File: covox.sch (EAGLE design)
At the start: 25 parts, among them CN1 POWERJACK, IC1 74HCT373N, IC2 74HC164N

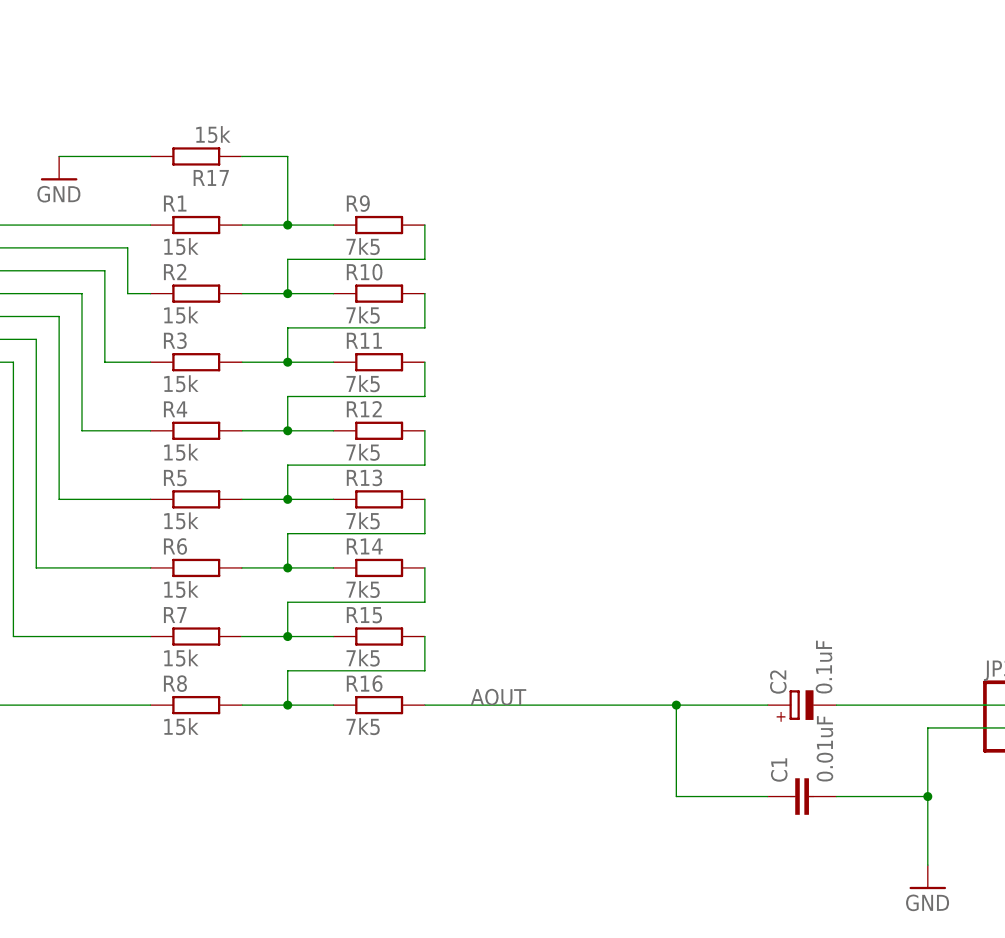
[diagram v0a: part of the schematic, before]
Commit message: Updates...
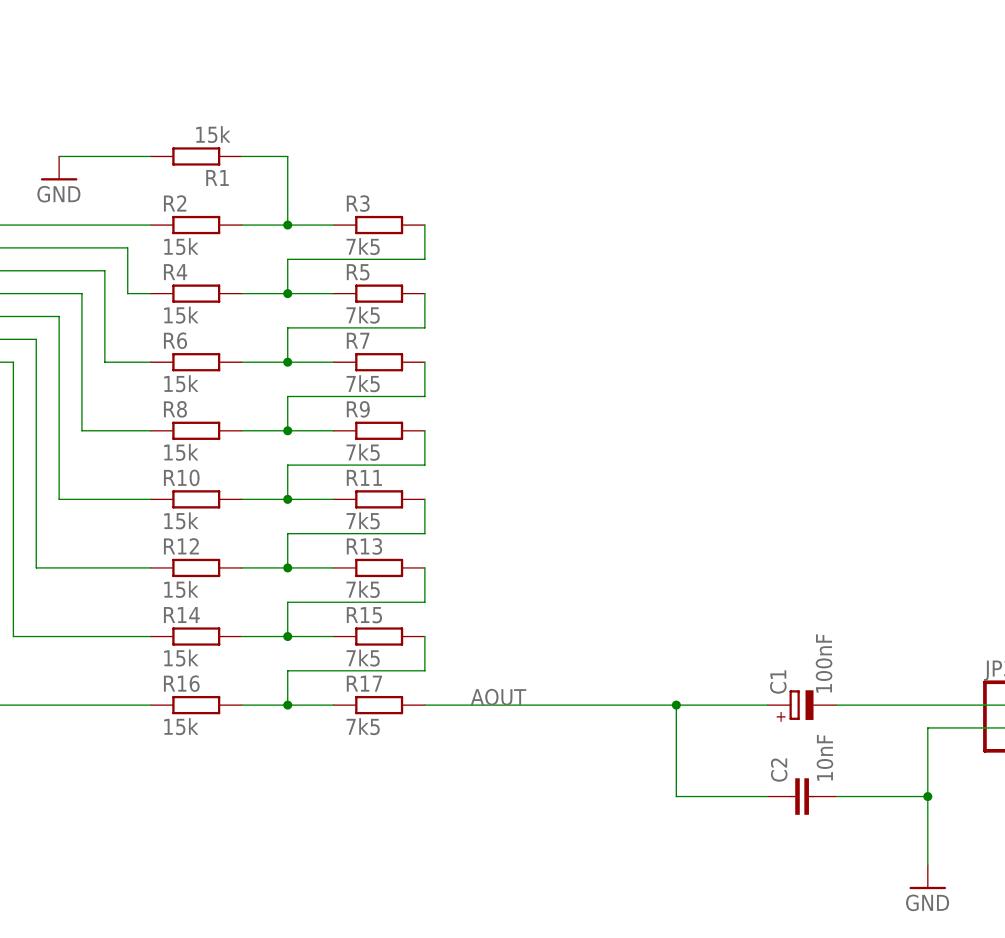
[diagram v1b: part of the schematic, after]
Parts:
- C1: value 0.01uF -> 100nF; device rcl:C-EU025-025X050 -> rcl:CPOL-EUE2-4
- C2: value 0.1uF -> 10nF; device rcl:CPOL-EUE2-4 -> rcl:C-EU025-025X050
- R10, R12, R14, R16: value 7k5 -> 15k
- R17, R3, R5, R7: value 15k -> 7k5
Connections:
- net AOUT: now also C1.+, C2.1, R17.2; no longer C1.1, C2.+, R16.2
- net GND: now also C2.2, R1.2; no longer C1.2, R17.2
- net N$1: now also R1.1, R2.2, R3.1; no longer R1.2, R17.1, R9.1
- net N$10: now also R6.1; no longer R3.1
- net N$11: now also R8.1; no longer R4.1
- net N$12: now also R10.1; no longer R5.1
- net N$13: now also R12.1; no longer R6.1
- net N$14: now also R14.1; no longer R7.1
- net N$15: now also R16.1; no longer R8.1
- net N$17: now also R16.2, R17.1; no longer R16.1, R8.2
- net N$2: now also R3.2, R4.2, R5.1; no longer R10.1, R2.2, R9.2
- net N$28: now also C1.-; no longer C2.-
- net N$3: now also R5.2, R6.2, R7.1; no longer R10.2, R11.1, R3.2
- net N$4: now also R7.2, R8.2, R9.1; no longer R11.2, R12.1, R4.2
- net N$5: now also R10.2, R11.1, R9.2; no longer R12.2, R13.1, R5.2
- net N$6: now also R11.2, R12.2, R13.1; no longer R13.2, R14.1, R6.2
- net N$7: now also R13.2; no longer R7.2
- net N$8: now also R2.1; no longer R1.1
- net N$9: now also R4.1; no longer R2.1
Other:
- moved on the sheet: R1, R10, R11, R12, R13, R14, R16, R17, R2, R3, R4, R5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
